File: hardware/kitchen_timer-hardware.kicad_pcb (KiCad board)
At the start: 2 copper layers, 60 x 110.8 mm, 80 parts, among them J1 Conn_01x02, J2 Conn_01x02_Pin, J3 AVR-ISP-6, Q1 JSM2302, Q2 IRLML6402, Q3 MMBT3904, SW2 SKRPACE010, U1 CH340E UART Module, U10 MAX7219, U11 KWM-20882CUYB, U12 KWM-20882CUYB, U13 KWM-20882CUYB, U14 KWM-20882CUYB, U2 TP4056 breakout, U3 SparkFun_LiPower, U5 ATMEGA328P-AU, U6 PEC11R-4215F-S0024, U7 MAX7219, U8 MAX7219, U9 MAX7219, Y1 Crystal-32kHz

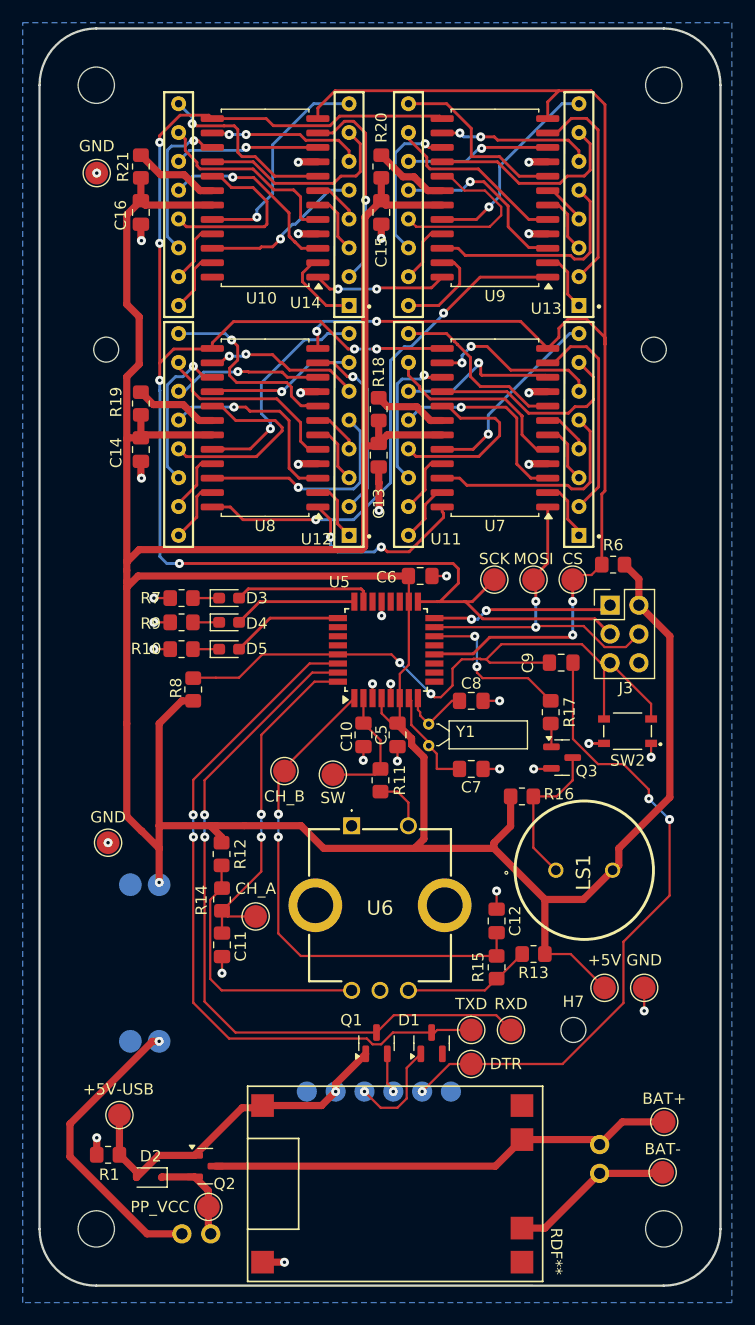
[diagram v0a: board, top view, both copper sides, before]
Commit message: Run "cleanup tracks and vias"
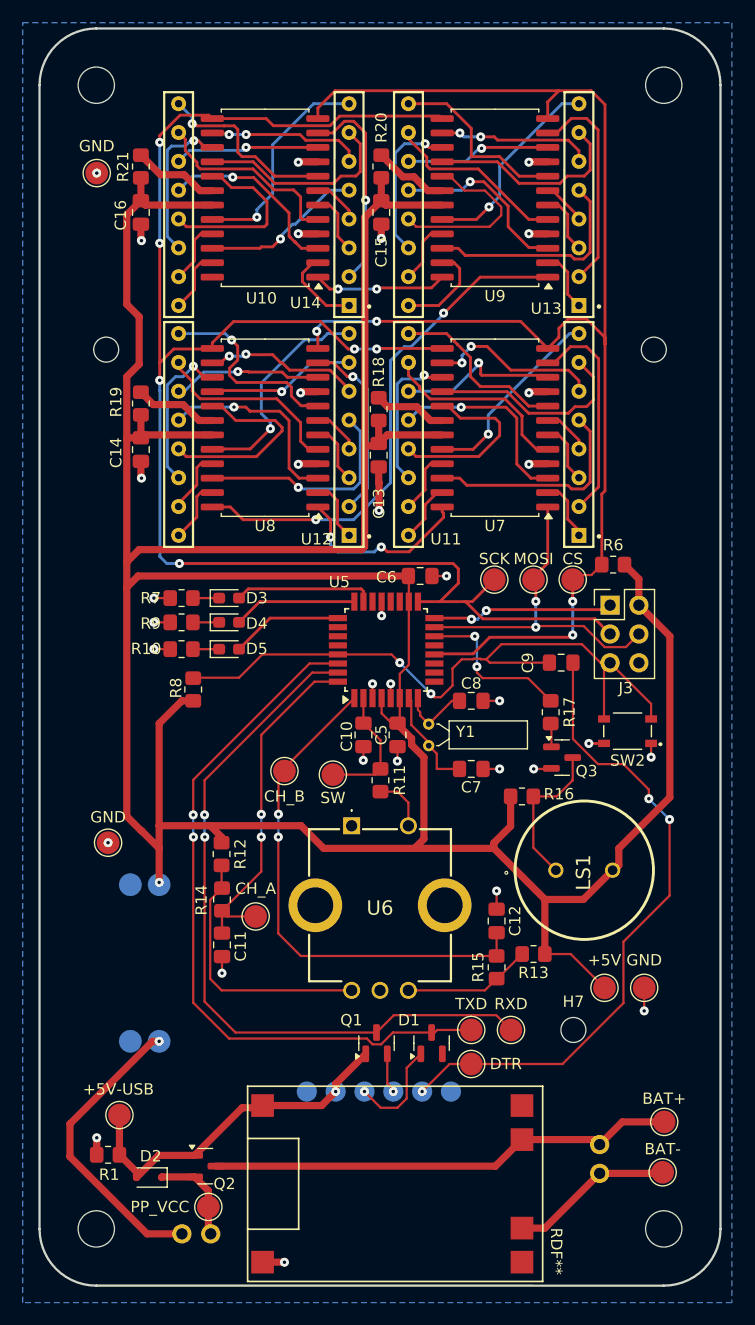
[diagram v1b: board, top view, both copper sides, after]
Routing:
- net /LED Matrices Drivers/SCK: track 144.2 -> 143.1 mm
- net /Microcontroller/SW: track 12.0 -> 11.3 mm
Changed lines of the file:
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@@
 	)
 	(segment
-		(start 161.5775 76.184)
-		(end 161.54 76.184)
-		(width 0.2)
-		(layer "F.Cu")
-		(net 1)
-	)
-	(segment
 		(start 151.523 59.944)
 		(end 150.1032 59.944)
@@
 	(segment
 		(start 160.04 100.184)
-		(end 163.04 100.184)
+		(end 167.04 100.184)
 		(width 0.635)
 		(layer "F.Cu")
@@
 	(segment
 		(start 134.6854 77.184)
-		(end 134.6854 76.684)
+		(end 134.6854 74.8792)
 		(width 0.635)
 		(layer "F.Cu")
@@
 	(segment
 		(start 134.6854 97.3582)
-		(end 134.6854 89.184)
+		(end 134.6854 77.184)
 		(width 0.635)
 		(layer "F.Cu")
@@
 	)
 	(segment
-		(start 163.04 100.184)
-		(end 167.04 100.184)
-		(width 0.635)
-		(layer "F.Cu")
-		(net 2)
-	)
-	(segment
 		(start 137.54 89.184)
 		(end 139.54 87.184)
@@
 	)
 	(segment
-		(start 142.54 98.184)
-		(end 145.04 98.184)
+		(start 142.04 98.184)
+		(end 150.04 98.184)
 		(width 0.635)
 		(layer "F.Cu")
@@
 	)
 	(segment
-		(start 142.04 98.184)
-		(end 142.54 98.184)
-		(width 0.635)
-		(layer "F.Cu")
-		(net 2)
-	)
-	(segment
 		(start 135.7776 53.34)
 		(end 134.6865 52.2489)
@@
 	)
 	(segment
-		(start 134.6854 75.684)
-		(end 134.6854 74.8792)
-		(width 0.635)
-		(layer "F.Cu")
-		(net 2)
-	)
-	(segment
 		(start 158.0025 89.1465)
 		(end 158.54 89.1465)
@@
 	)
 	(segment
-		(start 134.6854 89.184)
-		(end 134.6854 77.184)
-		(width 0.635)
-		(layer "F.Cu")
-		(net 2)
-	)
-	(segment
 		(start 173.8024 109.4952)
 		(end 171.5248 109.4952)
@@
 	)
 	(segment
-		(start 159.5935 78.3917)
-		(end 159.54 78.4452)
-		(width 0.2)
-		(layer "F.Cu")
-		(net 2)
-	)
-	(segment
-		(start 134.6854 76.684)
-		(end 134.6854 75.684)
-		(width 0.635)
-		(layer "F.Cu")
-		(net 2)
-	)
-	(segment
 		(start 135.93 64.008)
 		(end 136.184 63.754)
@@
 	)
 	(segment
-		(start 145.04 98.184)
-		(end 150.04 98.184)
-		(width 0.635)
-		(layer "F.Cu")
-		(net 2)
-	)
-	(segment
 		(start 158.74 88.9465)
 		(end 158.54 89.1465)
@@
 	)
 	(segment
-		(start 142.54 85.1465)
+		(start 141.0775 85.1465)
 		(end 144.5775 85.1465)
 		(width 0.2)
@@
 		(net 5)
 	)
-	(segment
-		(start 141.0775 85.1465)
-		(end 142.54 85.1465)
-		(width 0.2)
-		(layer "F.Cu")
-		(net 5)
-	)
 	(via
 		(at 161.4824 86.5632)
@@
 	)
 	(segment
-		(start 157.54 93.684)
-		(end 157.04 93.184)
-		(width 0.2)
-		(layer "F.Cu")
-		(net 7)
-	)
-	(segment
 		(start 157.04 90.6465)
 		(end 155.54 89.1465)
@@
 	)
 	(segment
-		(start 146.54 97.835)
-		(end 146.54 97.184)
-		(width 0.2)
-		(layer "B.Cu")
-		(net 8)
-	)
-	(segment
 		(start 146.54 99.184)
-		(end 146.54 97.835)
+		(end 146.54 97.184)
 		(width 0.2)
 		(layer "B.Cu")
@@
 	)
 	(segment
-		(start 161.544 116.4105)
-		(end 161.544 116.188)
-		(width 0.2)
-		(layer "F.Cu")
-		(net 10)
-	)
-	(segment
 		(start 140.54 113.7792)
 		(end 143.7024 116.9416)
@@
 	)
 	(segment
-		(start 140.536592 99.1015)
-		(end 140.54 99.104908)
-		(width 0.2)
-		(layer "F.Cu")
-		(net 10)
-	)
-	(segment
 		(start 161.544 116.4105)
 		(end 161.8135 116.4105)
@@
 	)
 	(segment
-		(start 155.555525 121.684)
-		(end 155.54 121.684)
-		(width 0.2)
-		(layer "F.Cu")
-		(net 11)
-	)
-	(segment
-		(start 155.630125 121.6094)
-		(end 155.555525 121.684)
-		(width 0.2)
-		(layer "F.Cu")
-		(net 11)
-	)
-	(segment
 		(start 160.594 118.2855)
 		(end 159.3488 119.5307)
@@
 		(net 11)
 	)
-	(segment
-		(start 155.630125 121.6094)
-		(end 155.640329 121.599196)
-		(width 0.2)
-		(layer "F.Cu")
-		(net 11)
-	)
 	(via
 		(at 155.630125 121.6094)
@@
 		(net 13)
 	)
-	(segment
-		(start 153.04 121.659525)
-		(end 153.090125 121.6094)
-		(width 0.635)
-		(layer "F.Cu")
-		(net 13)
-	)
 	(via
 		(at 153.090125 121.6094)
@@
 		(net 23)
 	)
-	(segment
-		(start 161.79 80.6952)
-		(end 161.893124 80.592076)
-		(width 0.2)
-		(layer "F.Cu")
-		(net 23)
-	)
 	(via
 		(at 170.728 78.4194)
@@
 	)
 	(segment
-		(start 162.04 78.4452)
+		(start 160.34 78.4452)
 		(end 162.2788 78.4452)
 		(width 0.254)
@@
 	)
 	(segment
-		(start 160.34 78.4452)
-		(end 162.04 78.4452)
-		(width 0.254)
-		(layer "F.Cu")
-		(net 24)
-	)
-	(segment
 		(start 147.5968 36.508)
 		(end 146.9688 35.88)
@@
 	)
 	(segment
-		(start 176.651 81.295)
-		(end 177.2704 81.295)
-		(width 0.254)
-		(layer "F.Cu")
-		(net 24)
-	)
-	(segment
 		(start 137.588 37.377757)
 		(end 137.588 37.971615)
@@
 	)
 	(segment
-		(start 156.7072 56.1848)
-		(end 156.312 56.1848)
-		(width 0.254)
-		(layer "F.Cu")
-		(net 24)
-	)
-	(segment
 		(start 162.2788 78.4452)
 		(end 164.4288 78.4452)
@@
 	)
 	(segment
-		(start 141.540003 97.231203)
-		(end 141.54 97.2312)
-		(width 0.2)
-		(layer "F.Cu")
-		(net 28)
-	)
-	(segment
-		(start 153.3012 84.684)
-		(end 153.29 84.6952)
-		(width 0.2)
-		(layer "F.Cu")
-		(net 28)
-	)
-	(segment
 		(start 141.54 94.184)
 		(end 151.0288 84.6952)
@@
 	)
 	(segment
-		(start 141.536594 99.101499)
-		(end 141.54 99.104905)
-		(width 0.2)
-		(layer "F.Cu")
-		(net 28)
-	)
-	(segment
 		(start 151.0288 84.6952)
 		(end 153.29 84.6952)
@@
 	)
 	(segment
-		(start 172.1025 91.234)
-		(end 172.05602 91.18752)
-		(width 0.2)
-		(layer "F.Cu")
-		(net 29)
-	)
-	(segment
 		(start 174.3856 76.0984)
 		(end 175.6256 76.0984)
@@
 	)
 	(segment
-		(start 169.458 109.4284)
-		(end 169.5248 109.4952)
-		(width 0.2)
-		(layer "F.Cu")
-		(net 33)
-	)
-	(segment
 		(start 159.5 112.6952)
 		(end 166.242 112.6952)
@@
 		(net 90)
 	)
-	(segment
-		(start 165.9499 38.505)
-		(end 165.9485 38.5064)
-		(width 0.254)
-		(layer "B.Cu")
-		(net 90)
-	)
